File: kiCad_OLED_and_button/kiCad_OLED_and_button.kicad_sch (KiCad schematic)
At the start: 6 parts, among them J1 OLED, J2 POWER and GND, J3 PICO pins, SW1 SW_Push, SW2 SW_Push, SW3 SW_Push

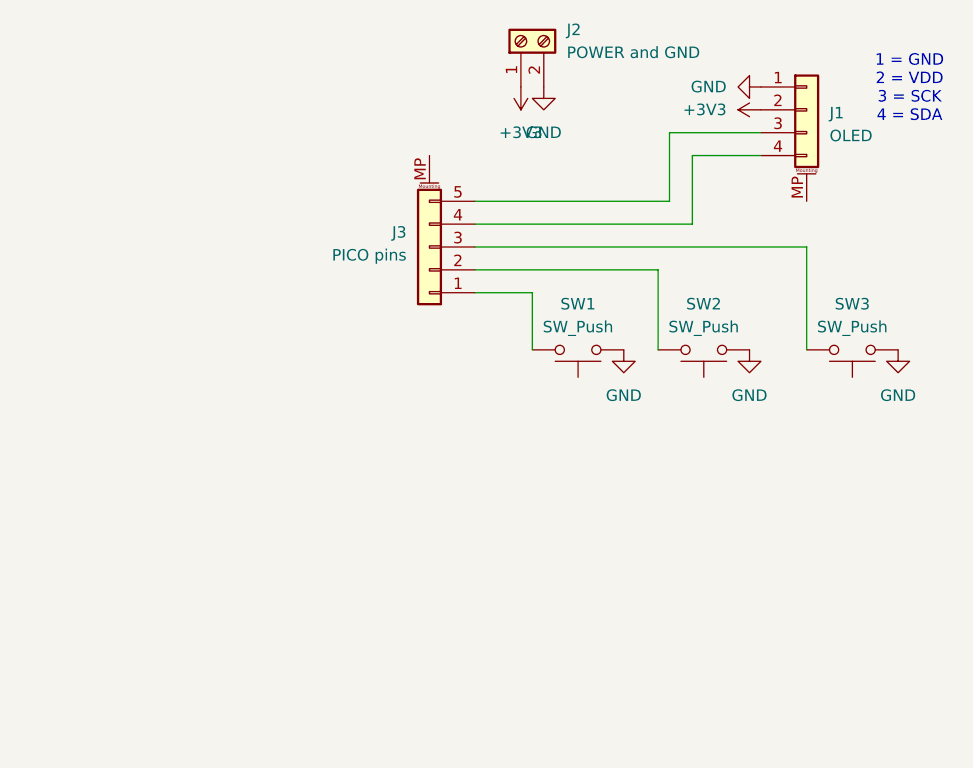
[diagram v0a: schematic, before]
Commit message: kicad stuuf idk
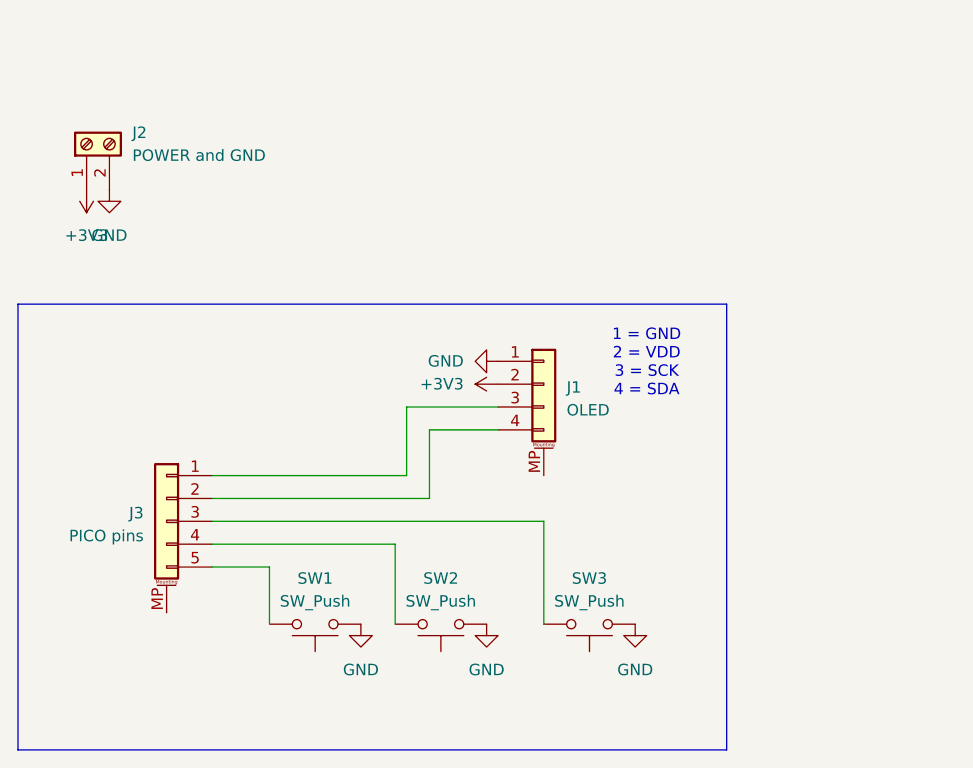
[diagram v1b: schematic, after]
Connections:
- net at J1.3 (SCK): now also J3.1 (Pin_1); no longer J3.5 (Pin_5)
- net at J1.4 (SDA): now also J3.2 (Pin_2); no longer J3.4 (Pin_4)
- net at SW1.2: now also J3.5 (Pin_5); no longer J3.1 (Pin_1)
- net at SW2.2: now also J3.4 (Pin_4); no longer J3.2 (Pin_2)
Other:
- moved on the sheet: J1, J2, J3, SW1, SW2, SW3
